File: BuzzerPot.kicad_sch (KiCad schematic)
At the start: 9 parts, among them J1 ConnM_01x03_Horizontal_2.54mm, U1 SC8002B

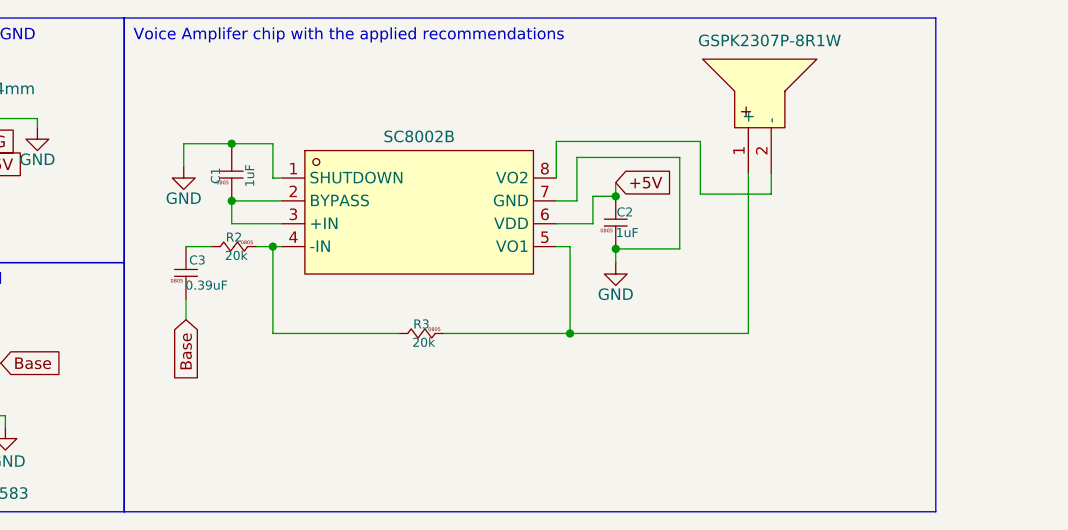
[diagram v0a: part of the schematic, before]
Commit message: Updated: Remal Golden Standard Recheck
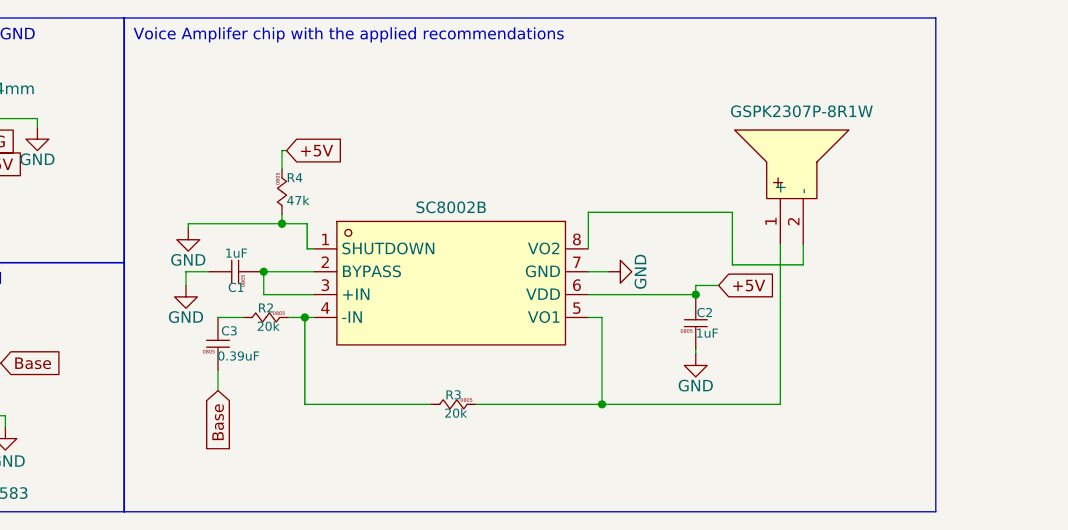
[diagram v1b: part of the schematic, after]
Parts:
- added R4: 47k, Remal_KiCadLib:R_0805_2012m, symbol Remal_KiCadLib:R_0805_2012m
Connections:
- net +5V: now also R4.2
- net GND: now also R4.1
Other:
- moved on the sheet: C1, C2, C3, R2, R3
